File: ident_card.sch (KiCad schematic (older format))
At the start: 4 parts

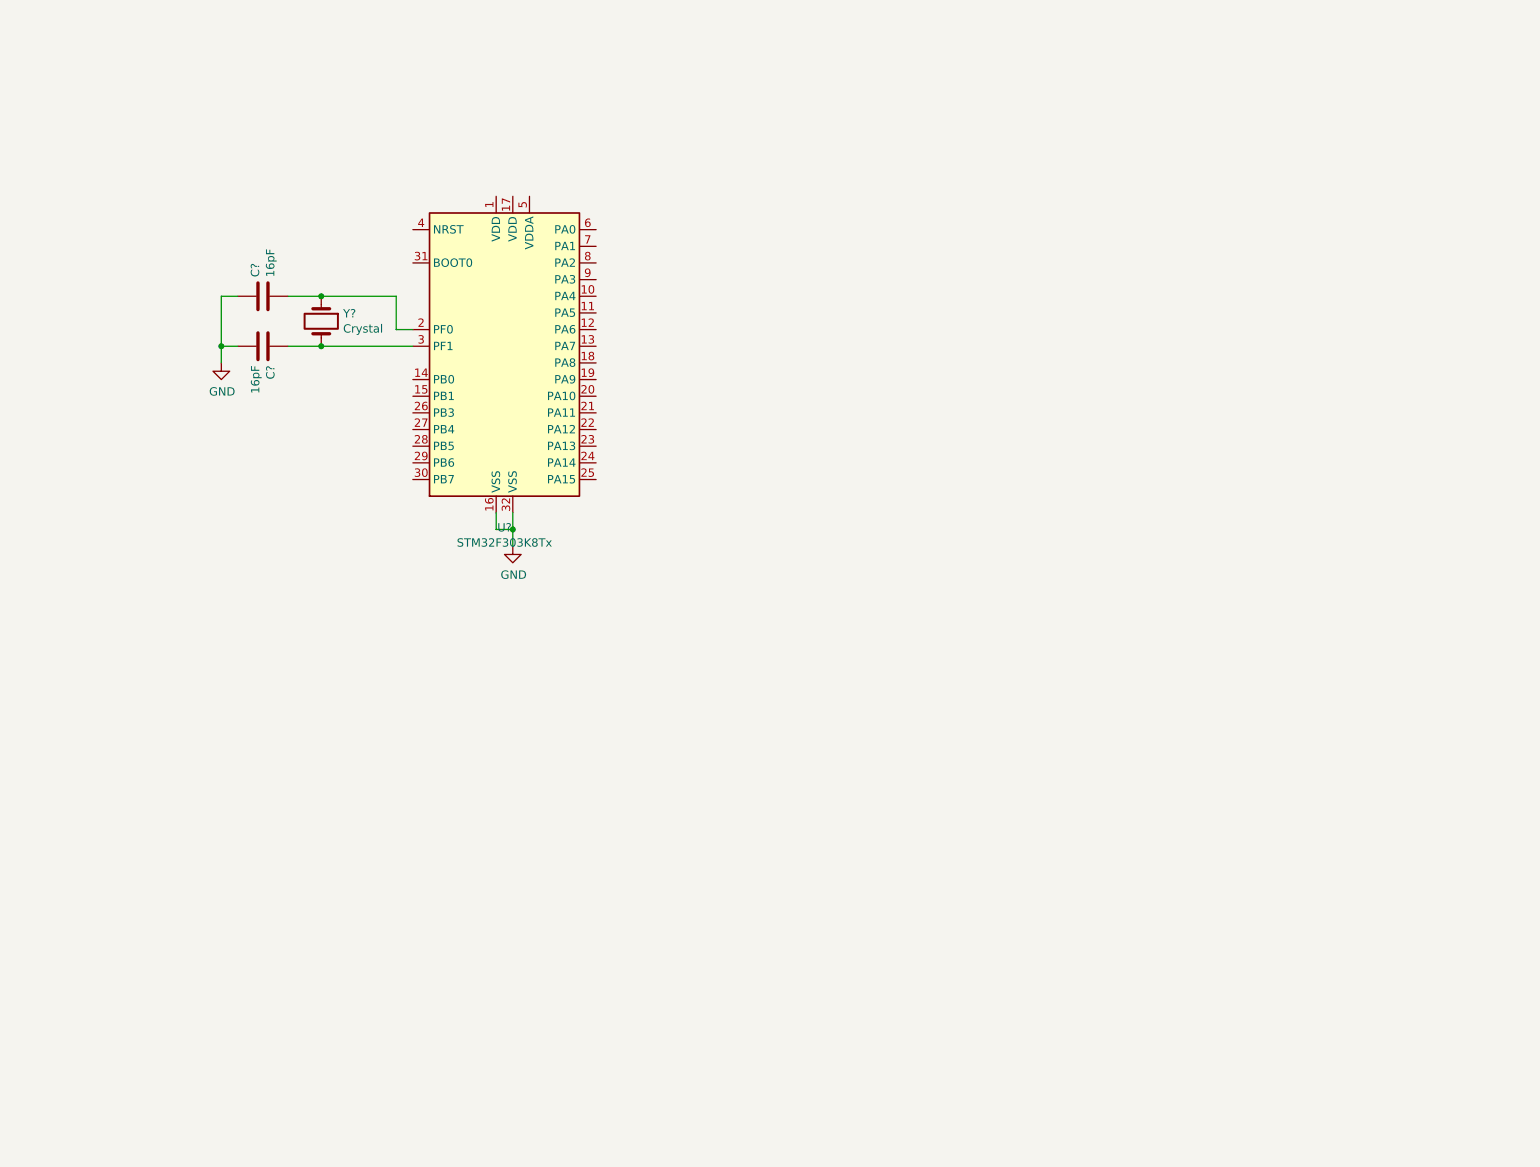
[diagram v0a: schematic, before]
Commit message: completed schematic
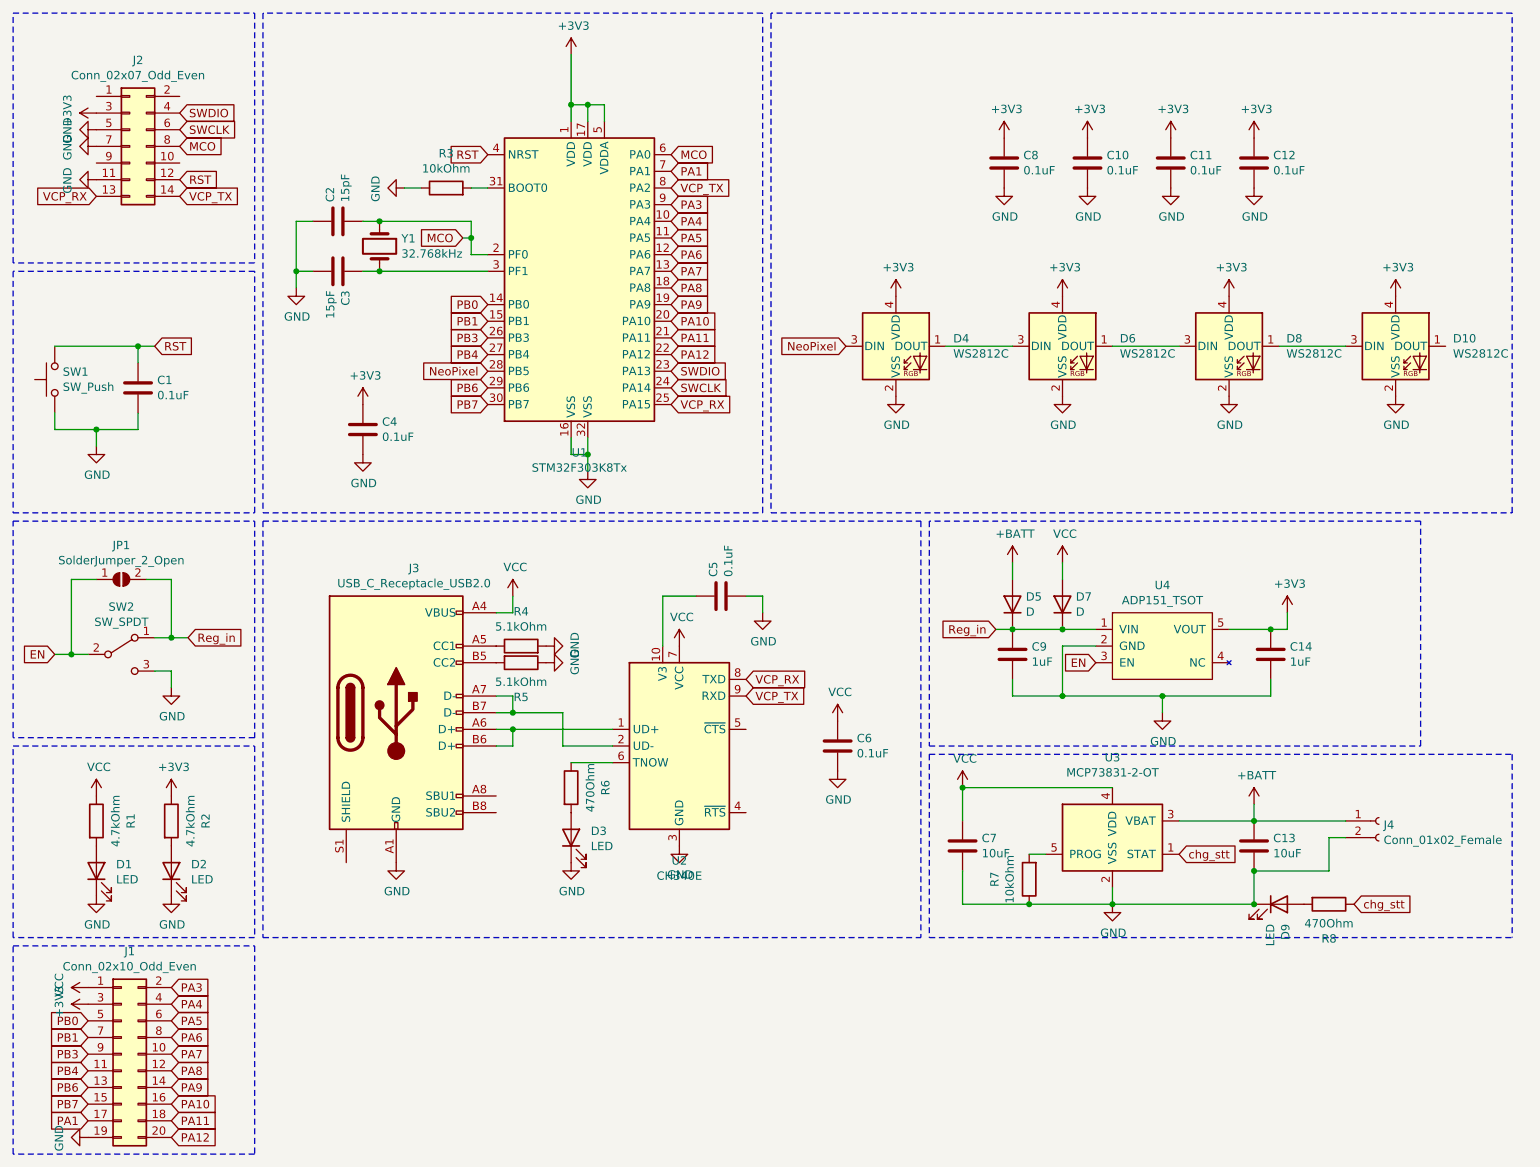
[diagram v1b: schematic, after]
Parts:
- added C1, C10, C11, C12, C4, C5, C6, C8: 0.1uF, Capacitor_SMD:C_0603_1608Metric, symbol Device:C
- added C13, C7: 10uF, Capacitor_SMD:C_0805_2012Metric, symbol Device:C
- added C14, C9: 1uF, Capacitor_SMD:C_0603_1608Metric, symbol Device:C
- added D1, D2, D3, D9: LED, LED_SMD:LED_0603_1608Metric, symbol Device:LED
- added D10, D4, D6, D8: WS2812C, LED_additional:LED_2020Metric_WS2812C_2.0x2.0mm_P1.0mm, symbol LED_additional:WS2812C
- added D5, D7: D, Diode_SMD:D_SOD-123F, symbol Device:D
- added J1: Conn_02x10_Odd_Even, Connector_PinHeader_2.54mm:PinHeader_2x10_P2.54mm_Vertical_SMD, symbol Connector_Generic:Conn_02x10_Odd_Even
- added J2: Conn_02x07_Odd_Even, Connector_PinHeader_1.27mm:PinHeader_2x07_P1.27mm_Vertical_SMD, symbol Connector_Generic:Conn_02x07_Odd_Even
- added J3: USB_C_Receptacle_USB2.0, Connector_USB:USB_C_Receptacle_HRO_TYPE-C-31-M-12, symbol Connector:USB_C_Receptacle_USB2.0
- added J4: Conn_01x02_Female, Connector_JST:JST_XA_S02B-XASK-1N-BN_1x02_P2.50mm_Horizontal, symbol Connector:Conn_01x02_Female
- added JP1: SolderJumper_2_Open, Jumper:SolderJumper-2_P1.3mm_Open_TrianglePad1.0x1.5mm, symbol Jumper:SolderJumper_2_Open
- added R1, R2: 4.7kOhm, Resistor_SMD:R_0603_1608Metric, symbol Device:R
- added R3, R7: 10kOhm, Resistor_SMD:R_0603_1608Metric, symbol Device:R
- added R4, R5: 5.1kOhm, Resistor_SMD:R_0603_1608Metric, symbol Device:R
- added R6, R8: 470Ohm, Resistor_SMD:R_0603_1608Metric, symbol Device:R
- added SW1: SW_Push, Button_Switch_additional:TVAF06-A020B-R, symbol Switch:SW_Push
- added SW2: SW_SPDT, Button_Switch_additional:IS-1245T-G, symbol Switch:SW_SPDT
- added U2: CH340E, Package_SO:MSOP-10_3x3mm_P0.5mm, symbol Interface_USB:CH340E
- added U3: MCP73831-2-OT, Package_TO_SOT_SMD:SOT-23-5, symbol Battery_Management:MCP73831-2-OT
- added U4: ADP151_TSOT, Package_TO_SOT_SMD:TSOT-23-5, symbol AnalogDevices:ADP151_TSOT
- C2, C3: renamed from C?; value 16pF -> 15pF; footprint (none) -> Capacitor_SMD:C_0603_1608Metric
- Y1: renamed from Y?; value Crystal -> 32.768kHz; footprint (none) -> Crystal_additional:Crystal_SMD_SeikoEpson_FC135-2Pin_3.2x1.5mm
- gave numbers to parts that had none: 1
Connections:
- net GND: now also C1.2, C10.2, C11.2, C12.2, C13.2, C14.2, C4.2, C5.2, C6.2, C7.2, C8.2, C9.2, D1.1 (K), D10.2 (VSS), D2.1 (K), D3.1 (K), D4.2 (VSS), D6.2 (VSS), D8.2 (VSS), D9.1 (K), J1.19 (Pin_19), J2.11 (Pin_11), J2.5 (Pin_5), J2.7 (Pin_7), J3.A1 (GND), J3.A12 (GND), J3.B1 (GND), J3.B12 (GND), J4.2 (Pin_2), R3.1, R4.2, R5.1, R7.1, SW1.1, SW2.3 (C), U2.3 (GND), U3.2 (VSS), U4.2 (GND)
- net +3V3: now reaches U1.1 (VDD)
- net +3V3: now also U1.17 (VDD), U1.5 (VDDA), C10.1, C11.1, C12.1, C14.1, C4.1, C8.1, D10.4 (VDD), D4.4 (VDD), D6.4 (VDD), D8.4 (VDD), J1.3 (Pin_3), J2.3 (Pin_3), R2.1, U4.5 (VOUT)
- net PA4: now reaches U1.10 (PA4)
- net PA4: now also J1.4 (Pin_4)
- net PA5: now reaches U1.11 (PA5)
- net PA5: now also J1.6 (Pin_6)
- net PA6: now reaches U1.12 (PA6)
- net PA6: now also J1.8 (Pin_8)
- net PA7: now reaches U1.13 (PA7)
- net PA7: now also J1.10 (Pin_10)
- net PB0: now reaches U1.14 (PB0)
- net PB0: now also J1.5 (Pin_5)
- net PB1: now reaches U1.15 (PB1)
- net PB1: now also J1.7 (Pin_7)
- net PA8: now reaches U1.18 (PA8)
- net PA8: now also J1.12 (Pin_12)
- net PA9: now reaches U1.19 (PA9)
- net PA9: now also J1.14 (Pin_14)
- net MCO: now reaches C2.2, U1.2 (PF0), Y1.1
- net MCO: now also U1.6 (PA0), J2.8 (Pin_8)
- net PA10: now reaches U1.20 (PA10)
- net PA10: now also J1.16 (Pin_16)
- net PA11: now reaches U1.21 (PA11)
- net PA11: now also J1.18 (Pin_18)
- net PA12: now reaches U1.22 (PA12)
- net PA12: now also J1.20 (Pin_20)
- net SWDIO: now reaches U1.23 (PA13)
- net SWDIO: now also J2.4 (Pin_4)
- net SWCLK: now reaches U1.24 (PA14)
- net SWCLK: now also J2.6 (Pin_6)
- net VCP_RX: now reaches U1.25 (PA15)
- net VCP_RX: now also J2.13 (Pin_13), U2.8 (TXD)
- net PB3: now reaches U1.26 (PB3)
- net PB3: now also J1.9 (Pin_9)
- net PB4: now reaches U1.27 (PB4)
- net PB4: now also J1.11 (Pin_11)
- net NeoPixel: now reaches U1.28 (PB5)
- net NeoPixel: now also D4.3 (DIN)
- net PB6: now reaches U1.29 (PB6)
- net PB6: now also J1.13 (Pin_13)
- net PB7: now reaches U1.30 (PB7)
- net PB7: now also J1.15 (Pin_15)
- net at U1.31 (BOOT0): now also R3.2
- net RST: now reaches U1.4 (NRST)
- net RST: now also C1.1, J2.12 (Pin_12), SW1.2
- net PA1: now reaches U1.7 (PA1)
- net PA1: now also J1.17 (Pin_17)
- net VCP_TX: now reaches U1.8 (PA2)
- net VCP_TX: now also J2.14 (Pin_14), U2.9 (RXD)
- net PA3: now reaches U1.9 (PA3)
- net PA3: now also J1.2 (Pin_2)
- new net: D4.1 (DOUT), D6.3 (DIN)
- new net: D6.1 (DOUT), D8.3 (DIN)
- new net: D10.3 (DIN), D8.1 (DOUT)
- new net: J3.A6 (D+), J3.B6 (D+), U2.1 (UD+)
- new net: C5.1, U2.10 (V3)
- new net: J3.A7 (D-), J3.B7 (D-), U2.2 (UD-)
- new net: R6.1, U2.6 (TNOW)
- new net: J3.A5 (CC1), R4.1
- new net: J3.B5 (CC2), R5.2
- new net: D3.2 (A), R6.2
- new net: R7.2, U3.5 (PROG)
- new net: D9.2 (A), R8.2
- new net: D1.2 (A), R1.2
- new net: D2.2 (A), R2.2
- new net +BATT: C13.1, D5.2 (A), J4.1 (Pin_1), U3.3 (VBAT)
- new net EN: JP1.1 (A), SW2.2 (B), U4.3 (EN)
- new net Reg_in: C9.1, D5.1 (K), D7.1 (K), JP1.2 (B), SW2.1 (A), U4.1 (VIN)
- new net VCC: C6.1, C7.1, D7.2 (A), J1.1 (Pin_1), J3.A4 (VBUS), J3.A9 (VBUS), J3.B4 (VBUS), J3.B9 (VBUS), R1.1, U2.7 (VCC), U3.4 (VDD)
- new net chg_stt: R8.1, U3.1 (STAT)
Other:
- moved on the sheet: C2, C3, U1, Y1
